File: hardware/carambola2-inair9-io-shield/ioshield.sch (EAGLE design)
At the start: 79 parts, among them IC1 PCF8591P, IC2 LM336LP, J1 I2C: RTC module, J10 RST, J12 Carambola2 J12, J13 Carambola2 J13, J2 22-23-2101, J3 inAir9-GND-wing, J4 inAir9 wing 2, J5 BMP180, J6 1Wire, J7 I2C, J8 USB, J9 Btn1

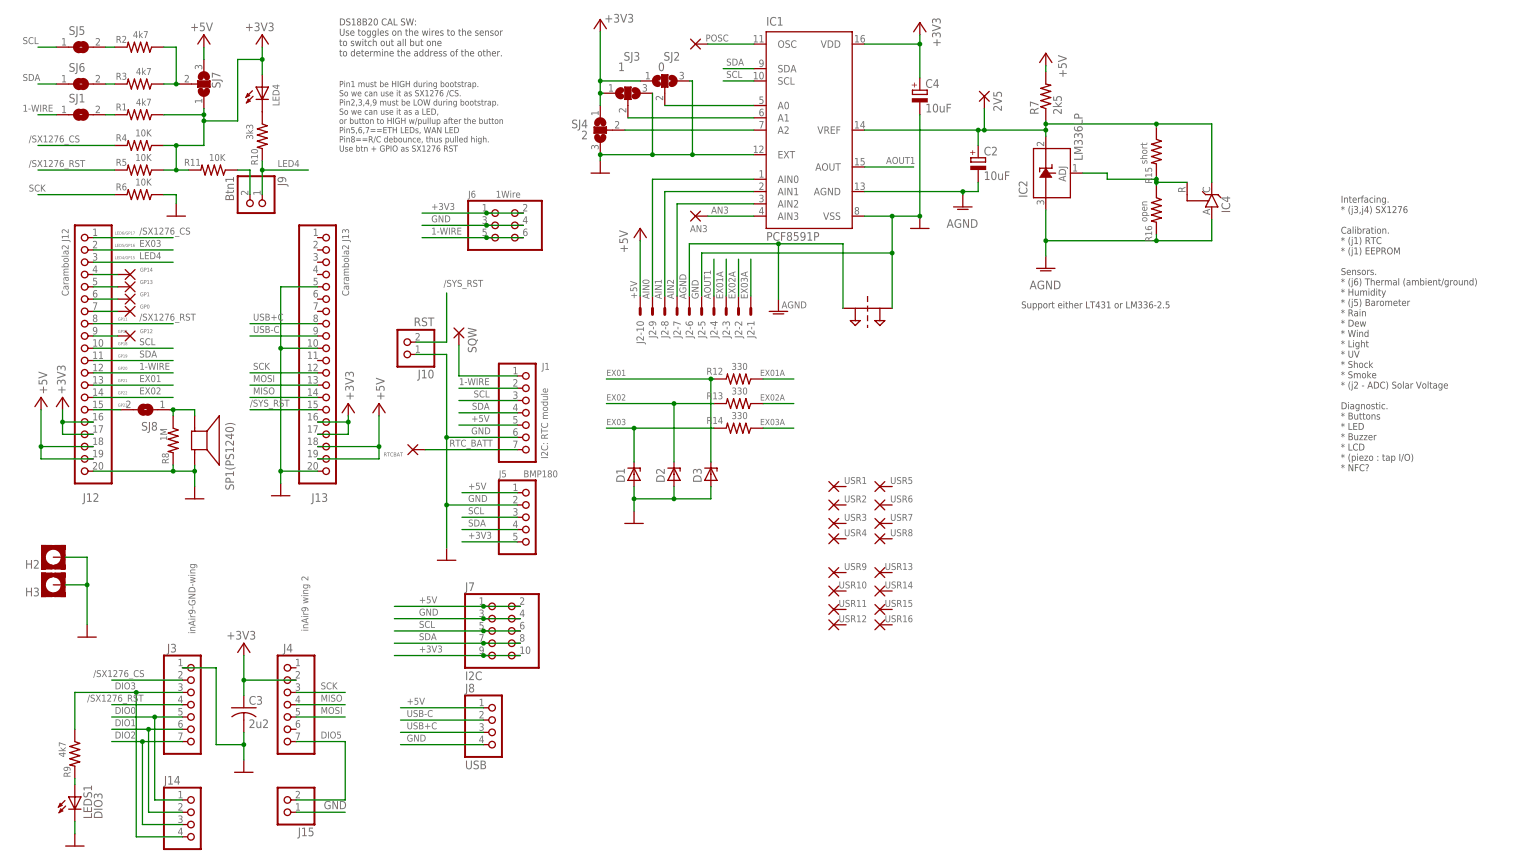
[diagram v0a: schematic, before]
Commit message: Schematics as provided to OshPark
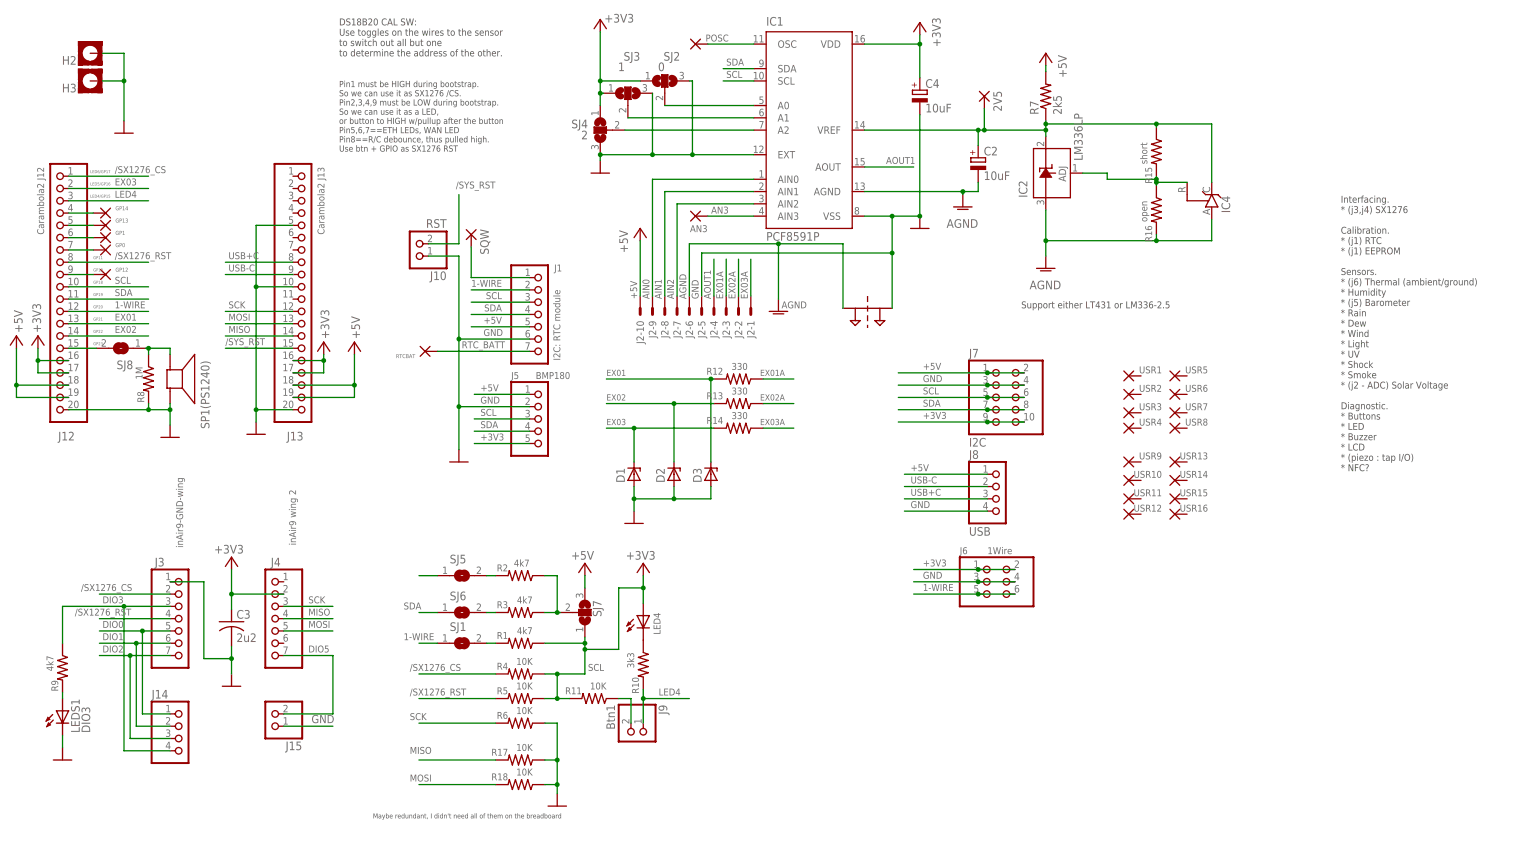
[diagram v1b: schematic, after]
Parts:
- added R17, R18: 10K, rcl:R-US_M1206
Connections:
- net GND: now also R17.1, R18.1
- net MISO: now also R17.2
- net MOSI: now also R18.2
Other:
- note added: "Maybe redundant, I didn't need all of them on the breadboard"
- moved on the sheet: C3, GP0, GP1, GP12, GP13, GP14, H2, H3, J1, J10, J12, J13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
